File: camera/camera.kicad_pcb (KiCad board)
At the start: 4 copper layers, 45.2 x 32.5 mm, 79 parts, among them J1 Gecko, J2 USB_B_Micro, J3 Programmer, J4 OV5640, J5 Micro_SD_Card, U1 INA180, U2 TPS562200, U3 MCP2562, U4 STM32H750VBTx, U5 TLV70215_SOT23-5, U6 AP2171W, X1 ECS-2520MV-240-BN

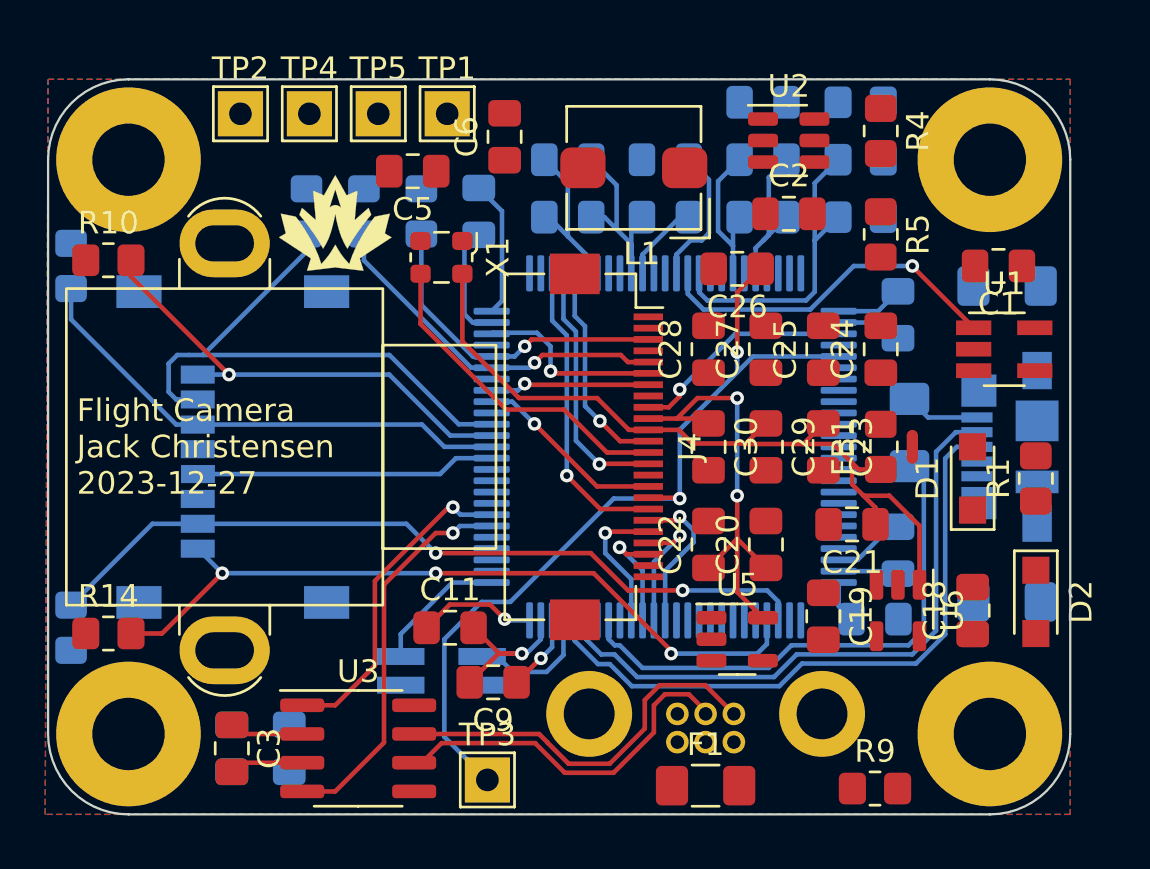
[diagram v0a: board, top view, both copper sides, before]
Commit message: Complete routing, ready for review
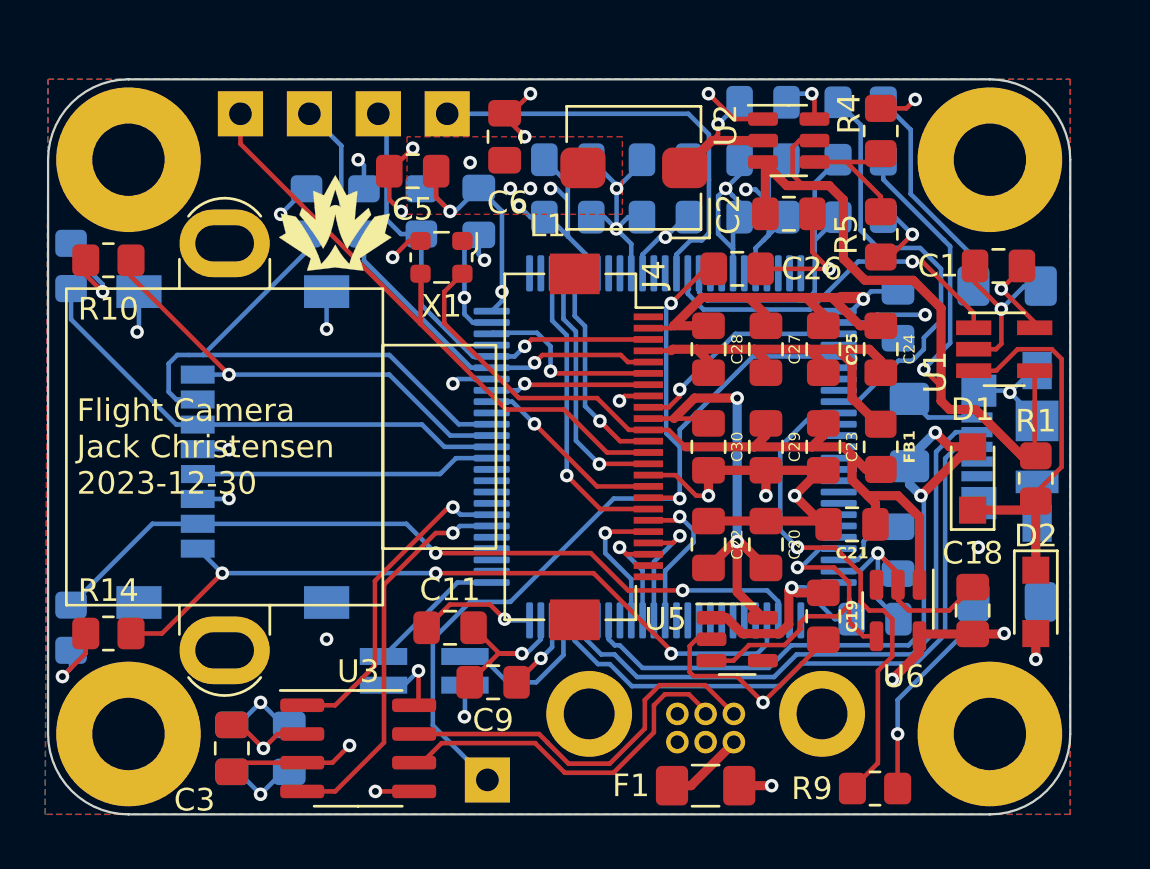
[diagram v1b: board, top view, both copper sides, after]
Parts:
- TP1, TP2, TP3, TP4, TP5: moved to B.Cu
- moved NT1 7.12 mm to (191.5, 93.5), turned to 180 degrees
- moved J3 0.76 mm to (172.6, 110.0)
- turned C26 to 0 degrees
- turned TP1 to 180 degrees
- turned TP2 to 180 degrees
- turned TP3 to 180 degrees
- turned TP4 to 180 degrees
- turned TP5 to 180 degrees
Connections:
- U4 pad 47: unconnected-(U4-PB11-Pad47) -> /MCU/CAM_EN
- U4 pad 97: /MCU/CAM_EN -> unconnected-(U4-PE0-Pad97)
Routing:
- net GND: track 38.3 -> 129.1 mm, vias 1 -> 32
- net +2V8: track 33.9 -> 87.5 mm, vias 1 -> 24
- net VDC: track 0.00 -> 42.5 mm, vias 0 -> 1
- net /MCU/LED_G: track 0.00 -> 22.4 mm, vias 0 -> 1
- net /OV5640/AVDD: track 0.00 -> 19.1 mm
- net +5V: track 3.28 -> 22.3 mm, vias 0 -> 1
- net /MCU/LED_R: track 0.00 -> 18.9 mm
- net Net-(D2-A): track 0.00 -> 17.6 mm, vias 0 -> 2
- net Net-(D1-K): track 0.00 -> 17.2 mm
- net GNDA: track 0.00 -> 16.8 mm
- net /MCU/CAM_EN: track 0.00 -> 15.5 mm, vias 0 -> 1
- net Net-(U4-NRST): track 6.28 -> 20.2 mm
- net /OV5640/XCLK: track 14.7 -> 27.2 mm
- net Net-(D3-A): track 0.00 -> 9.78 mm
- net Net-(D4-A): track 0.00 -> 9.64 mm, vias 0 -> 1
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- added copper zone on F.Cu, net +2V8
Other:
- board text added: "Flight Camera Jack Christensen 2023-12-30"
- board text removed: "Flight Camera Jack Christensen 2023-12-27"
